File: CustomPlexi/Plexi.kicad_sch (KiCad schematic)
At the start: 21 parts, among them U1 TL074

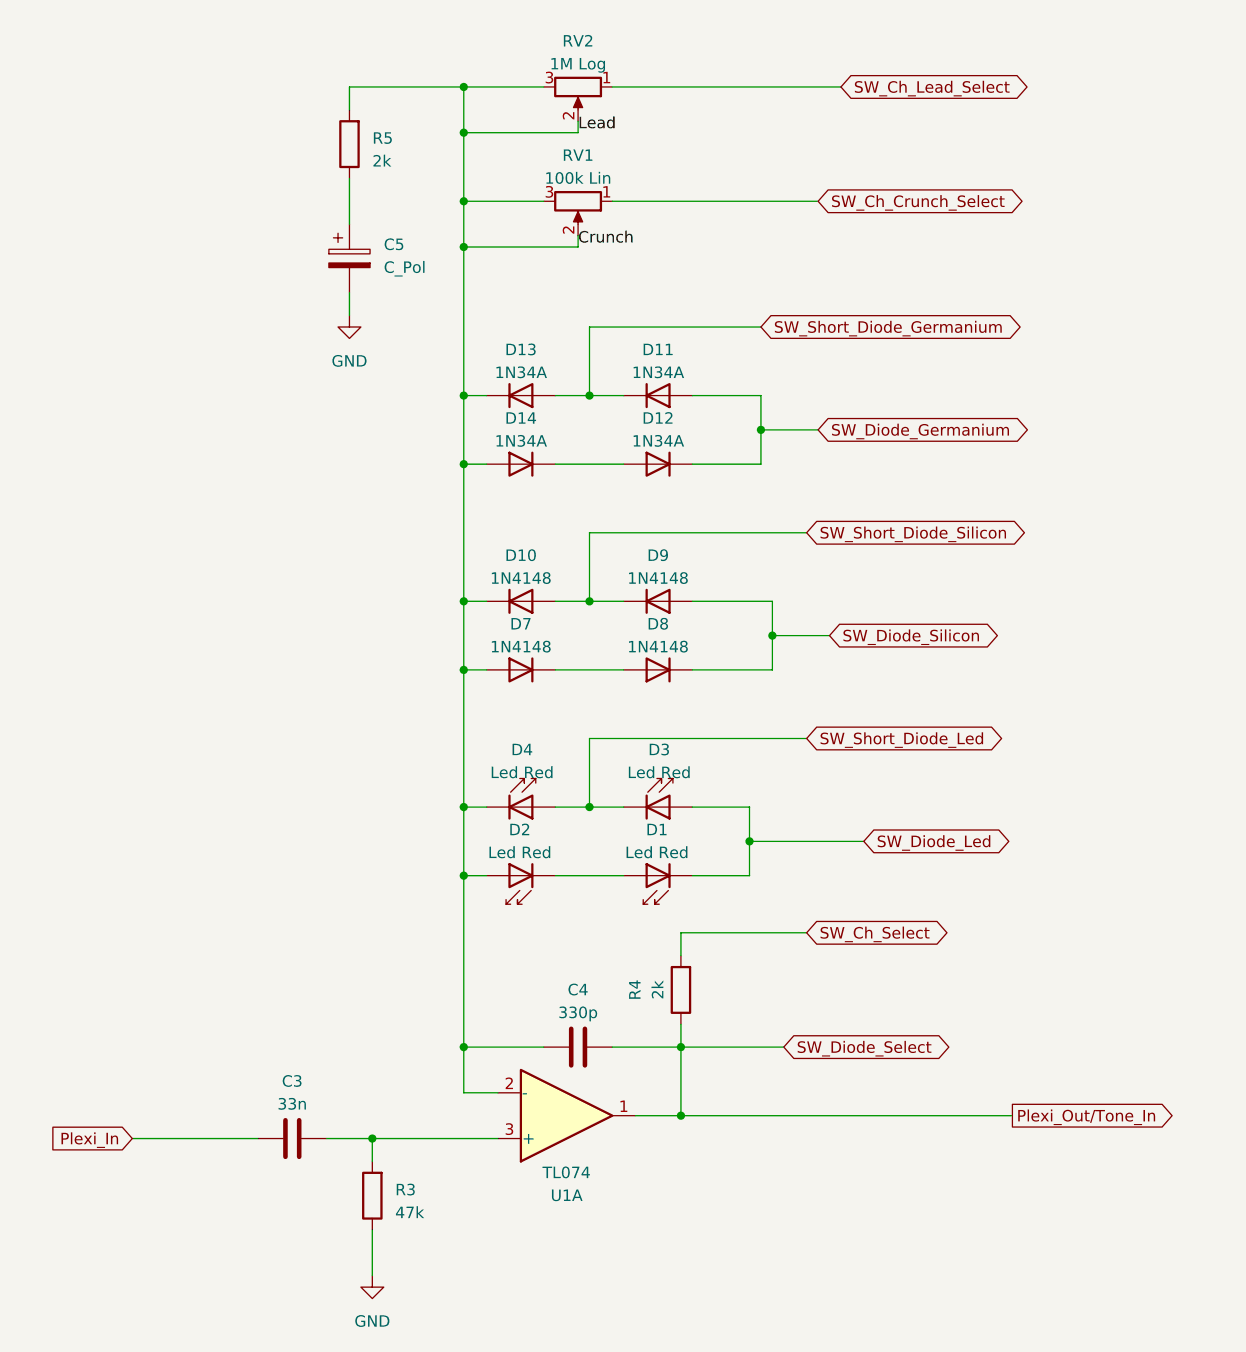
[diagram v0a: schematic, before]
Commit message: some changes
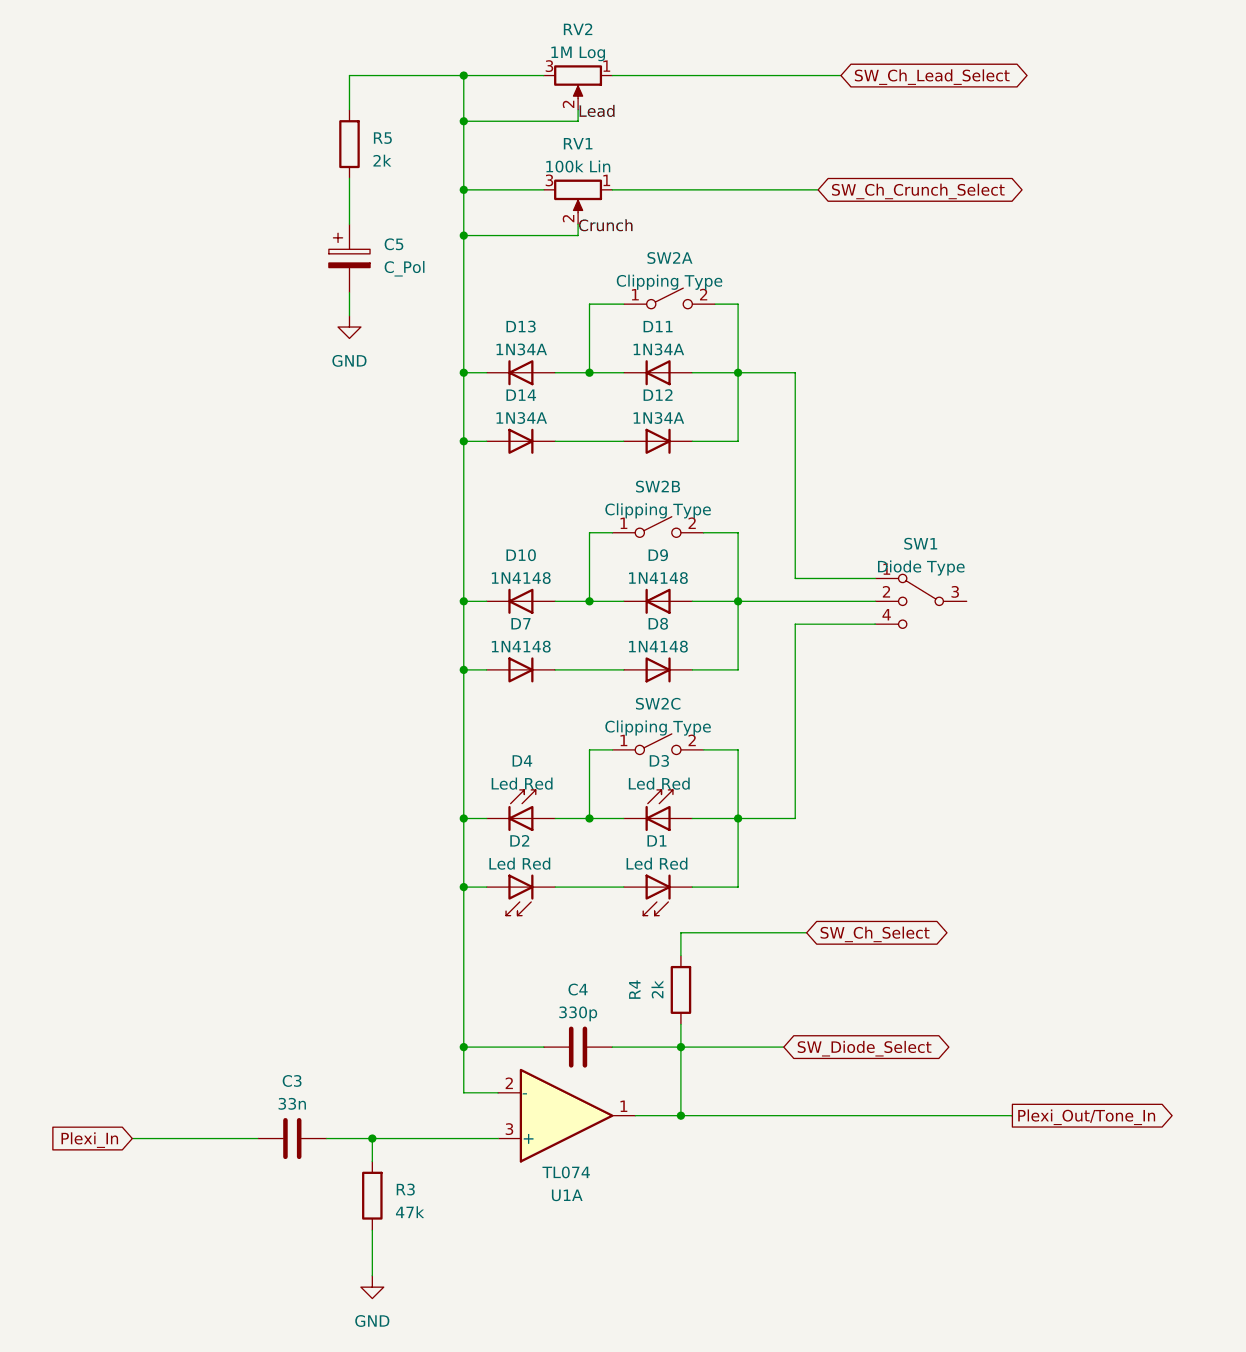
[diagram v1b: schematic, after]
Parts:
- added SW1: Diode Type, symbol Switch:SW_SP3T
- added SW2: Clipping Type, symbol CustomLib:SW_SPST_x3
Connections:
- net SW_Diode_Germanium: no longer names the net of D11.2 (A), D12.1 (K)
- net SW_Diode_Germanium: now also SW1.1, SW2.2
- net SW_Diode_Led: no longer names the net of D1.1 (K), D3.2 (A)
- net SW_Diode_Led: now also SW1.4, SW2.2
- net SW_Diode_Silicon: no longer names the net of D8.1 (K), D9.2 (A)
- net SW_Diode_Silicon: now also SW1.2, SW2.2
- net SW_Short_Diode_Germanium: no longer names the net of D11.1 (K), D13.2 (A)
- net SW_Short_Diode_Germanium: now also SW2.1
- net SW_Short_Diode_Led: no longer names the net of D3.1 (K), D4.2 (A)
- net SW_Short_Diode_Led: now also SW2.1
- net SW_Short_Diode_Silicon: no longer names the net of D10.2 (A), D9.1 (K)
- net SW_Short_Diode_Silicon: now also SW2.1
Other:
- moved on the sheet: D1, D11, D12, D13, D14, D2, D3, D4, RV1, RV2

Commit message: commit
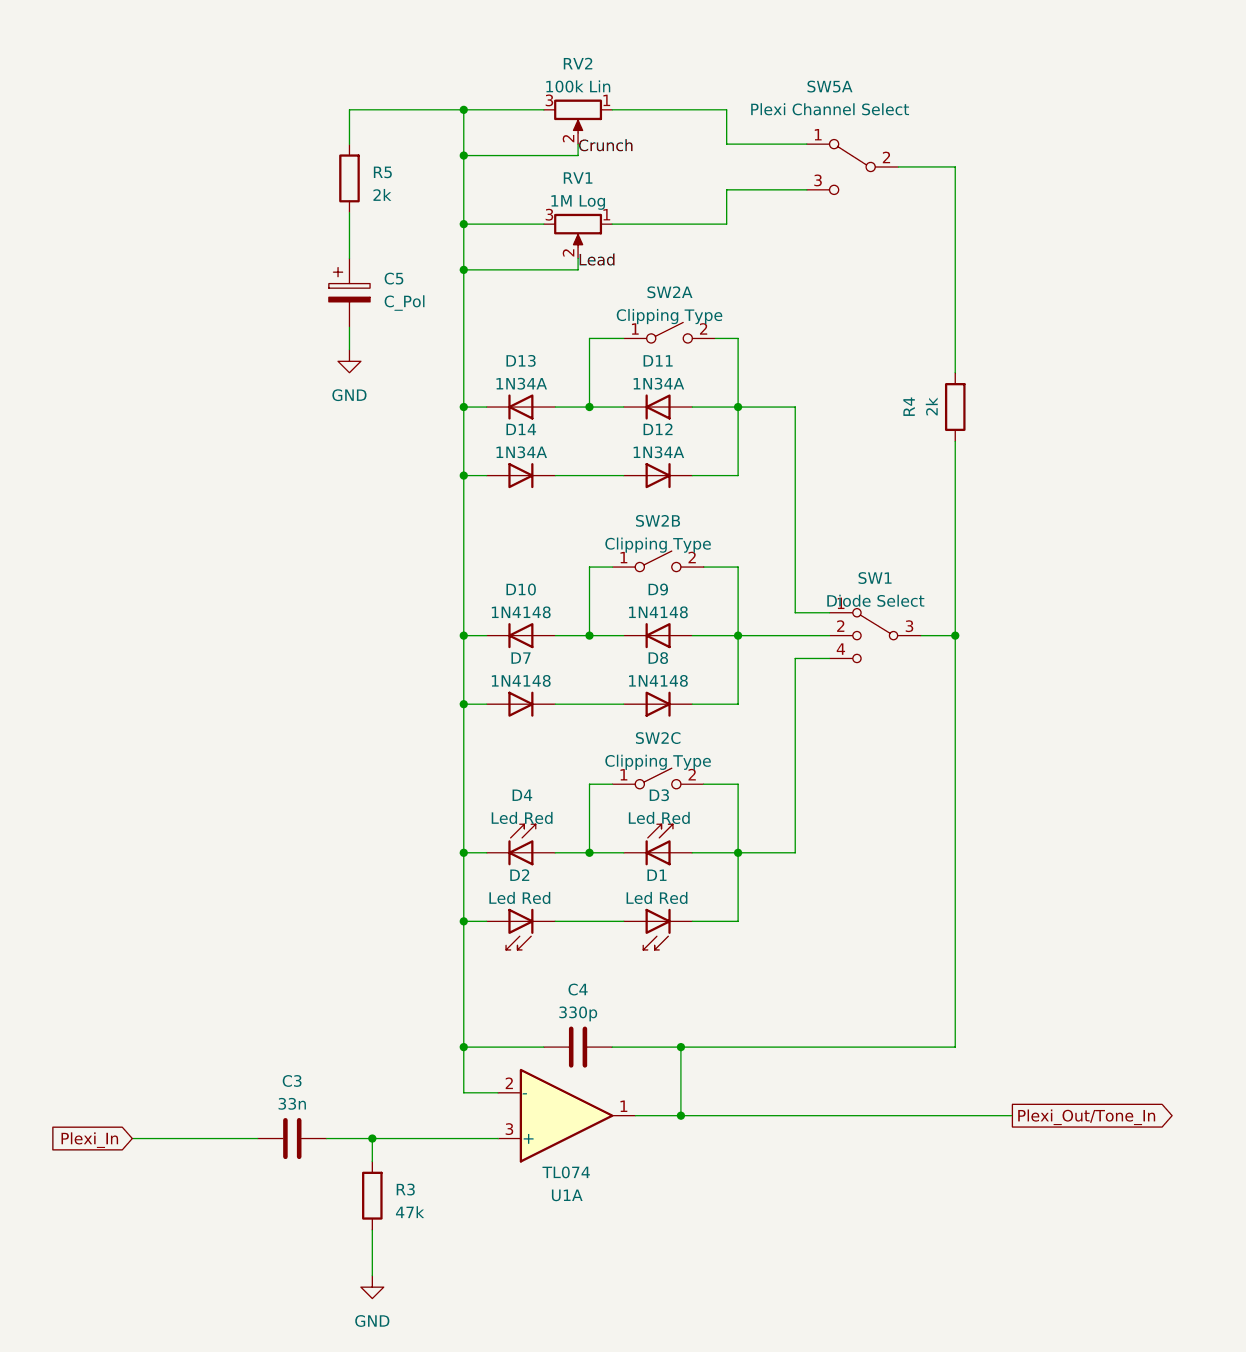
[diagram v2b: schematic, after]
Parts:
- added SW5: Plexi Channel Select, symbol CustomLib:SW_SPDT_x4
- RV1: value 100k Lin -> 1M Log
- RV2: value 1M Log -> 100k Lin
- SW1: value Diode Type -> Diode Select
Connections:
- net Plexi_Out/Tone_In: now also SW1.3
- net SW_Ch_Crunch_Select: no longer names the net of RV1.1
- net SW_Ch_Crunch_Select: now also SW5.3
- net SW_Ch_Lead_Select: no longer names the net of RV2.1
- net SW_Ch_Lead_Select: now also SW5.1
- net SW_Ch_Select: no longer names the net of R4.2
- net SW_Ch_Select: now also SW5.2
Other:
- moved on the sheet: C5, D1, D10, D11, D12, D13, D14, D2, D3, D4, D7, D8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
